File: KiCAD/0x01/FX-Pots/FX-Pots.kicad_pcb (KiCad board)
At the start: 2 copper layers, 100 x 100 mm, 41 parts, among them J1 IN, J2 OUT, SW1 SW_Push_LED, SW2 SW_Push_LED, SW3 SW_Push_LED, SW4 SW_Push_LED, SW5 SW_Push_LED, SW6 SW_Push_LED, SW7 SW_Push_LED, SW8 SW_Push_LED, U1 ADS7830, U2 HT16K33 24SOP

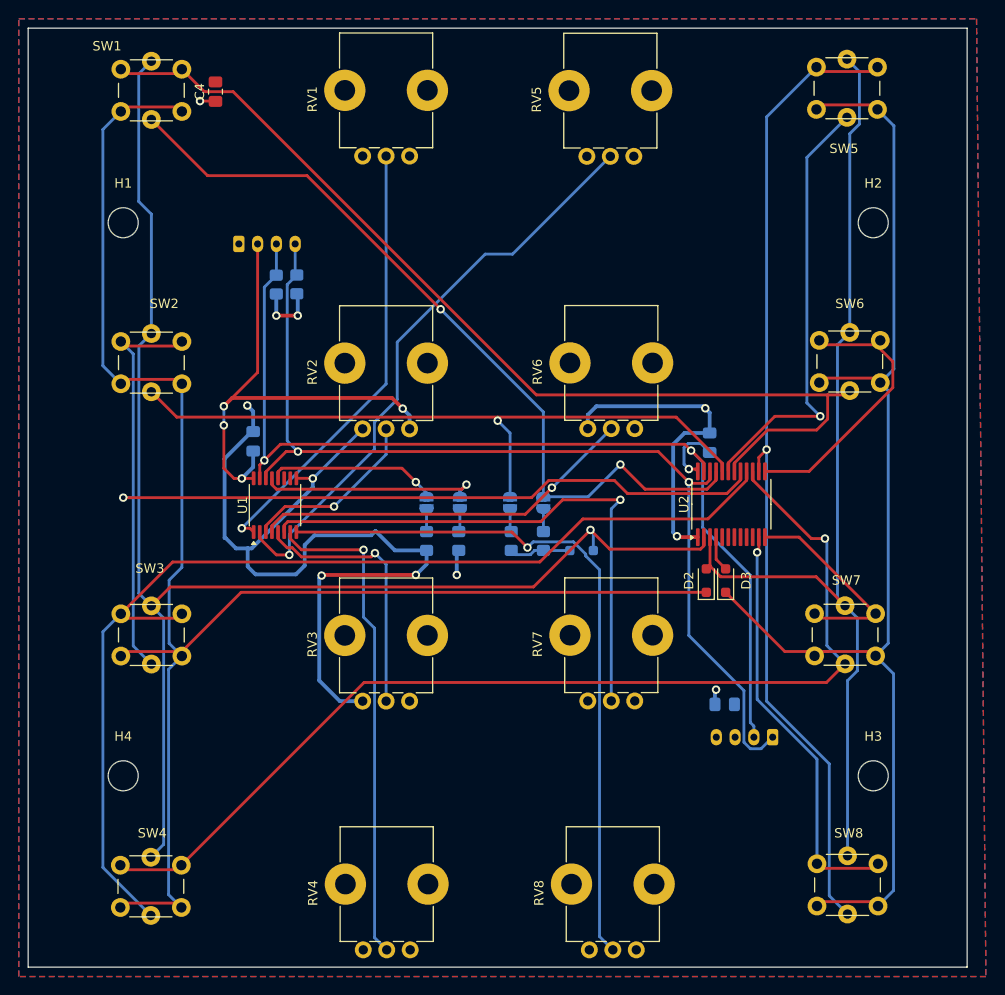
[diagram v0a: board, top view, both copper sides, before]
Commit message: step models
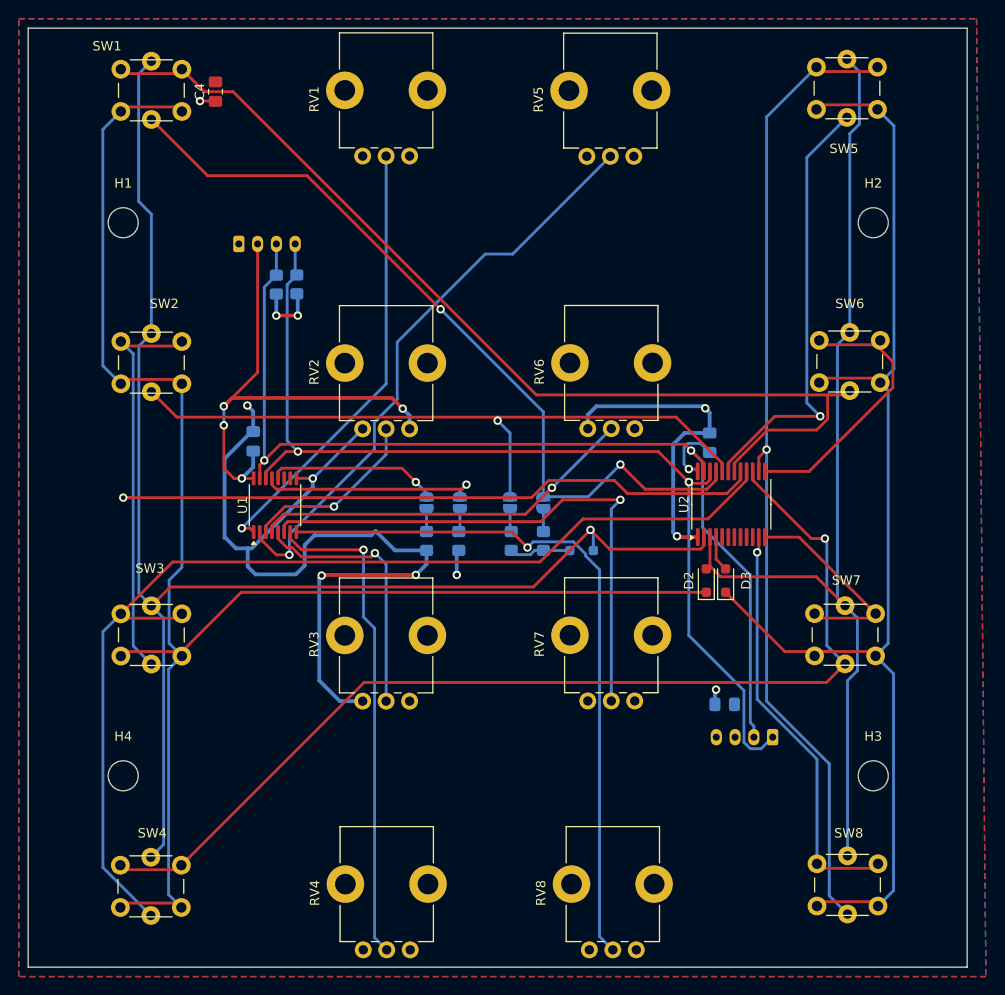
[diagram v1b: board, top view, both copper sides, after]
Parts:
- RV1, RV2, RV3, RV4, RV5, RV6, RV7, RV8: footprint Potentiometer_THT:Potentiometer_Bourns_PTV09A-1_Single_Vertical -> led-sw:Potentiometer_Bourns_PTV09A-1_Single_Vertical
